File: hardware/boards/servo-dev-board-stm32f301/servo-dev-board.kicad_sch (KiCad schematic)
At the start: 39 parts, among them J1 USB_B_Micro, J2 Conn_01x05_MountingPin, J3 Conn_01x04_MountingPin, J4 Conn_01x04_MountingPin, J5 Conn_02x05_Odd_Even, SW1 SW_Push, SW2 SW_Push, U1 DRV8231ADSGR, U2 SSP7615-33DFR, U3 STM32F301K8Ux, Y1 16MHz 9pF

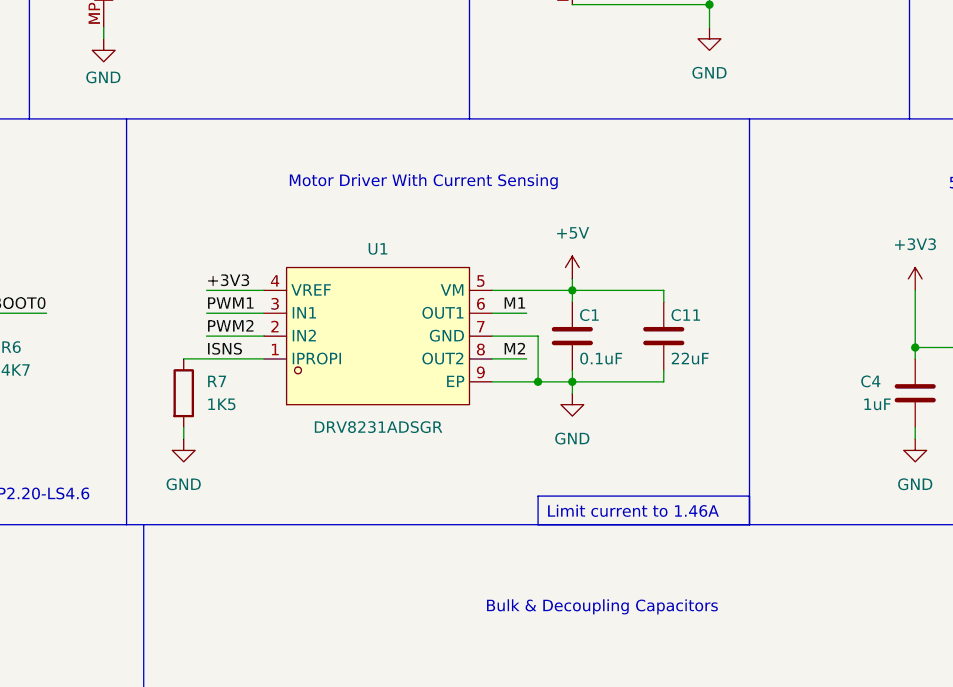
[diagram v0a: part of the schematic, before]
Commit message: re-organize shared folders
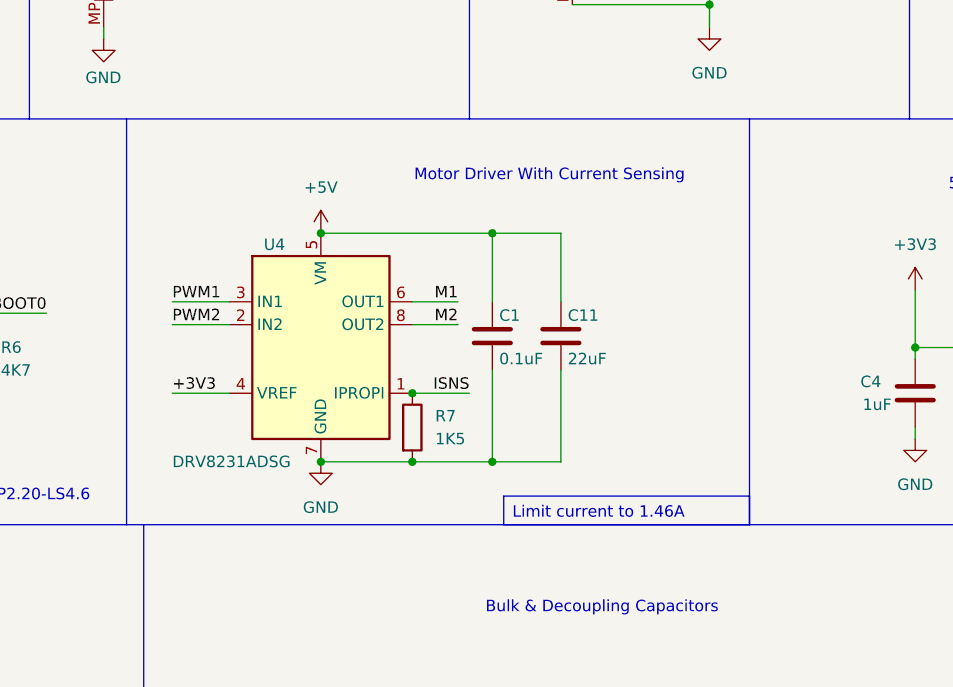
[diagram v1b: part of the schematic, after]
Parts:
- removed U1: DRV8231ADSGR, Package_SON:WSON-8-1EP_2x2mm_P0.5mm_EP0.9x1.6mm, symbol lib:DRV8231ADSGR
- added U4: DRV8231ADSG, Package_SON:WSON-8-1EP_2x2mm_P0.5mm_EP0.9x1.6mm, symbol Driver_Motor:DRV8231ADSG
- J5: footprint lib:IDC-TH_10P-P1.27-X1270WV-2X05A-6TV01 -> shared:IDC-TH_10P-P1.27-X1270WV-2X05A-6TV01
- U2: symbol lib:SSP7615-33DFR -> shared:SSP7615-33DFR
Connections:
- net +3V3: now also U4.4 (VREF)
- net +5V: now also U4.5 (VM)
- net GND: now also U4.7 (GND), U4.9 (GND)
- net ISNS: now also U4.1 (IPROPI)
- net M1: now also U4.6 (OUT1)
- net M2: now also U4.8 (OUT2)
- net PWM1: now also U4.3 (IN1)
- net PWM2: now also U4.2 (IN2)
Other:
- moved on the sheet: C1, C11, R7
